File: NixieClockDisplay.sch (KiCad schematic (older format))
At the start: 54 parts, among them J1 CONN_01X08, J2 CONN_01X03, U1 TPIC6B595, U2 TPIC6B595, U3 TPIC6B595, U4 TPIC6B595, U5 TPIC6B595, U6 TPIC6B595, U7 WE-FDSM_DC/DC_5V

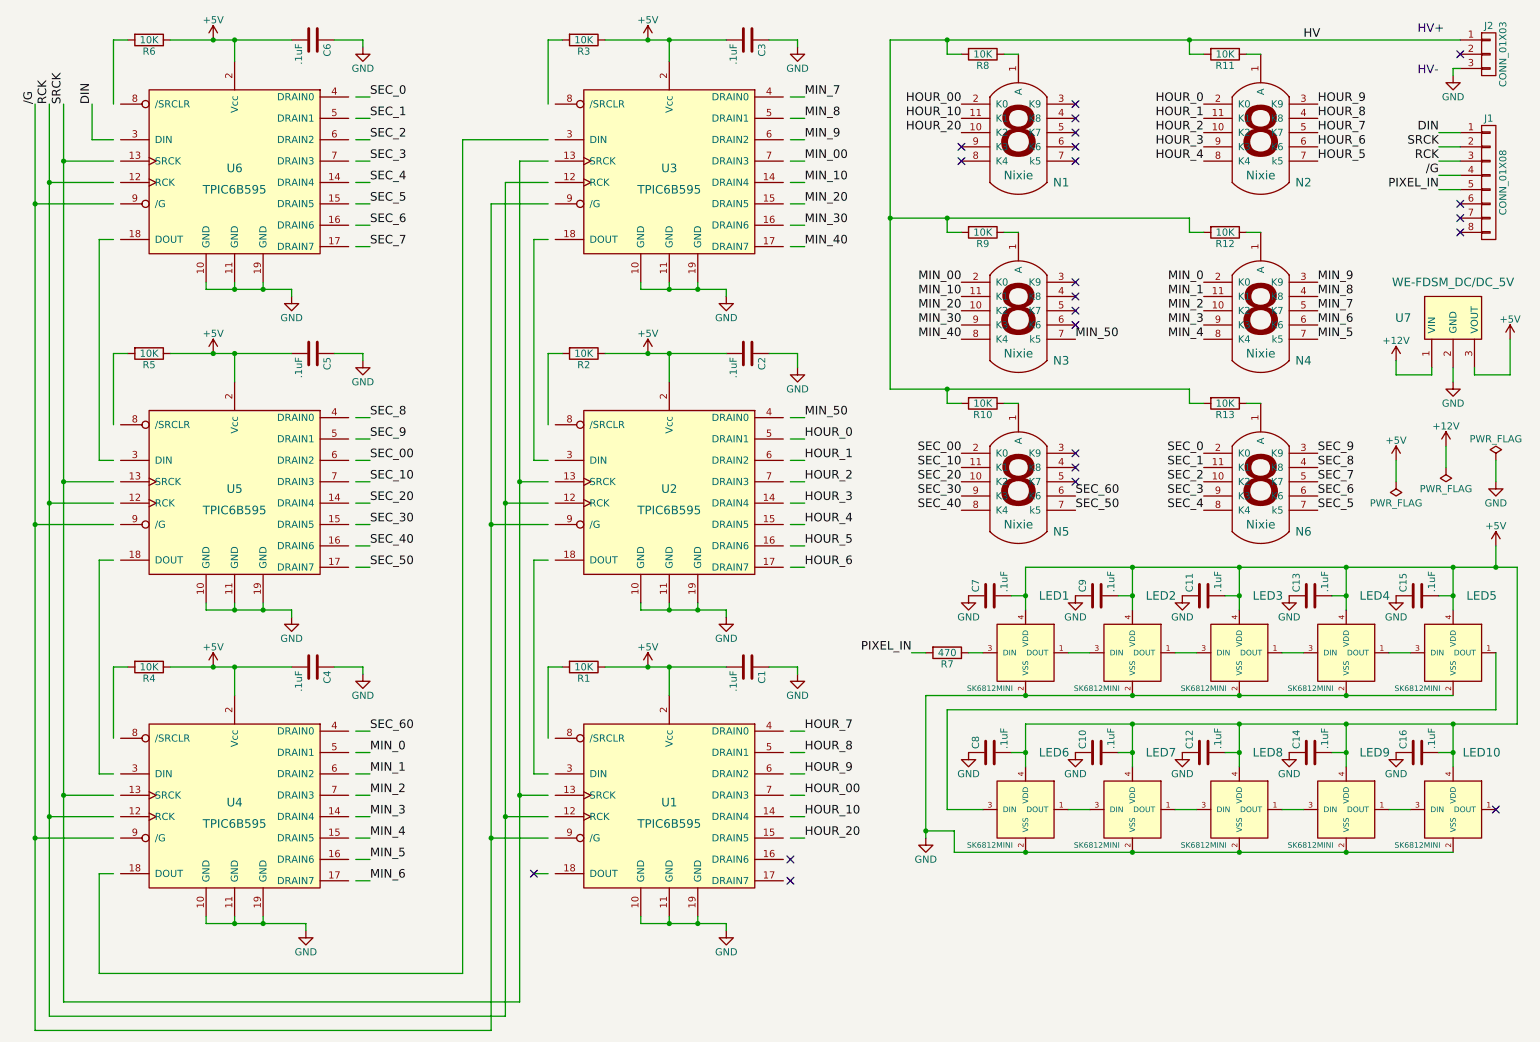
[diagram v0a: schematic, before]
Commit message: More layout
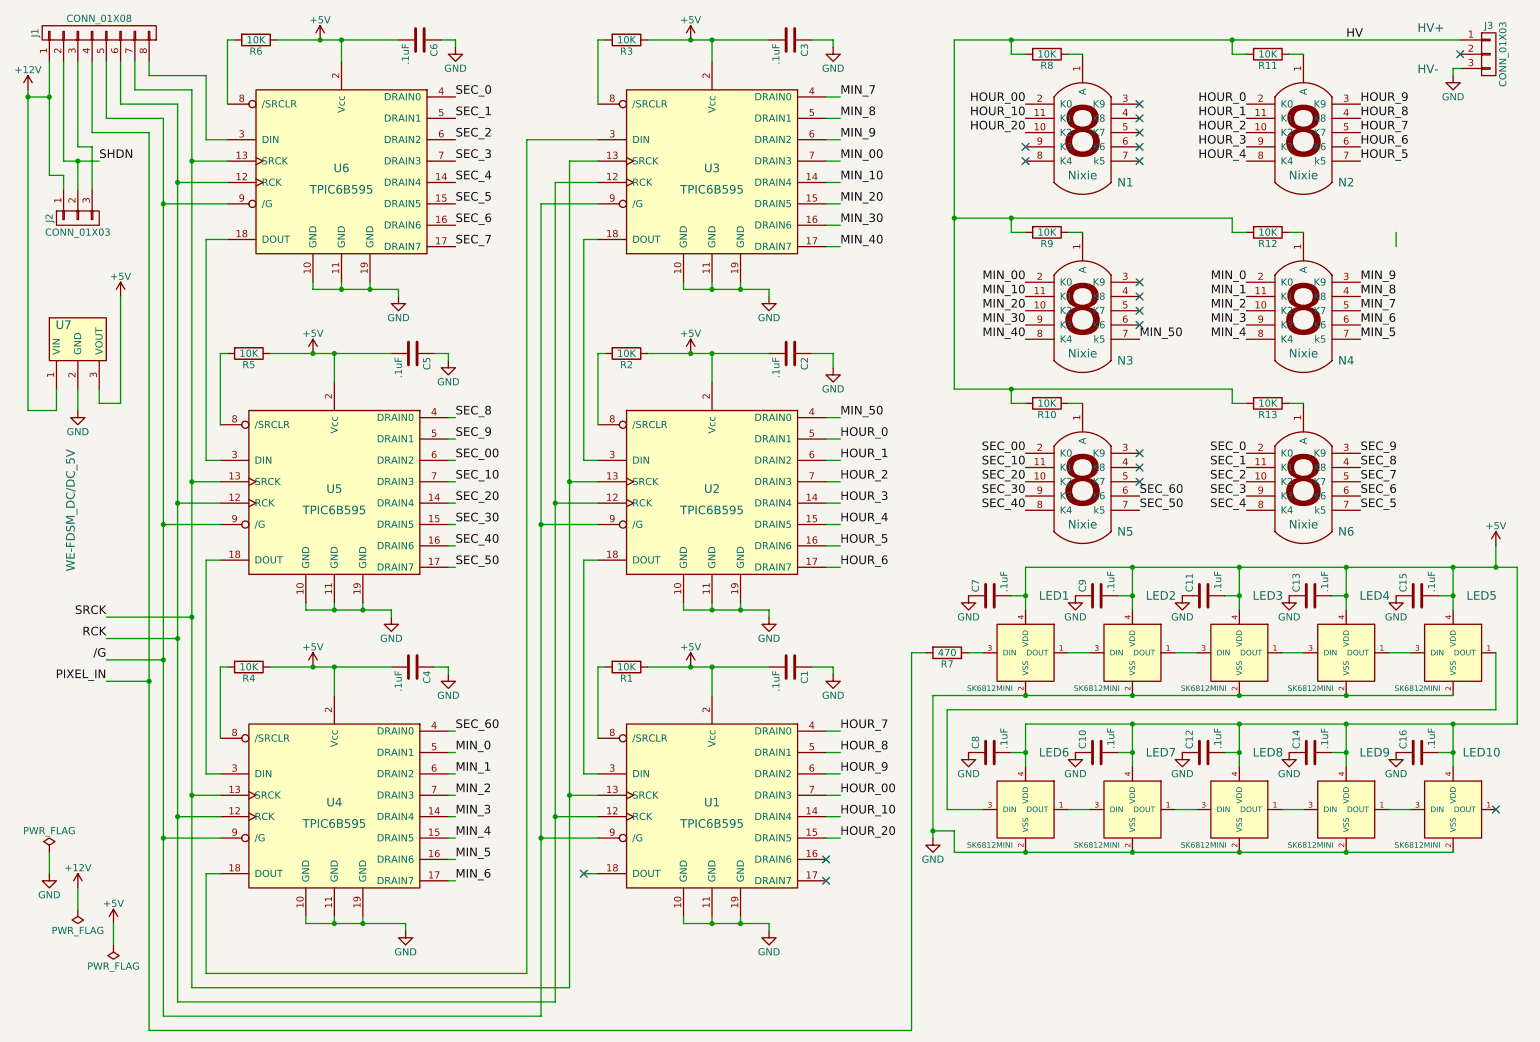
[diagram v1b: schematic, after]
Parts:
- added J2: CONN_01X03, Pin_Headers:Pin_Header_Angled_1x03_Pitch2.54mm, symbol CONN_01X03
- J1: footprint (none) -> Pin_Headers:Pin_Header_Angled_1x08_Pitch2.54mm
- J3: renamed from J2; footprint (none) -> Pin_Headers:Pin_Header_Angled_1x03_Pitch2.54mm
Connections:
- net labels added: SHDN
- net labels removed: DIN
- wire segments 241 -> 264
- no-connect marks 22 -> 19
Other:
- moved on the sheet: C1, C2, C3, C4, C5, C6, J1, N1, N2, N3, N4, N5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
